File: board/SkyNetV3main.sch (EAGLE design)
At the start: 61 parts, among them IC1 HC_05, IC2 RF4463PRO, IC3 LPC1768, IC4 BCX17, IC5 TPS63001, IC6 MCP73871-2CCI/ML, Q1 32.768KHz, Q2 12MHz, Q3 IRLM6402, Q4 BSS138, X1 BAT

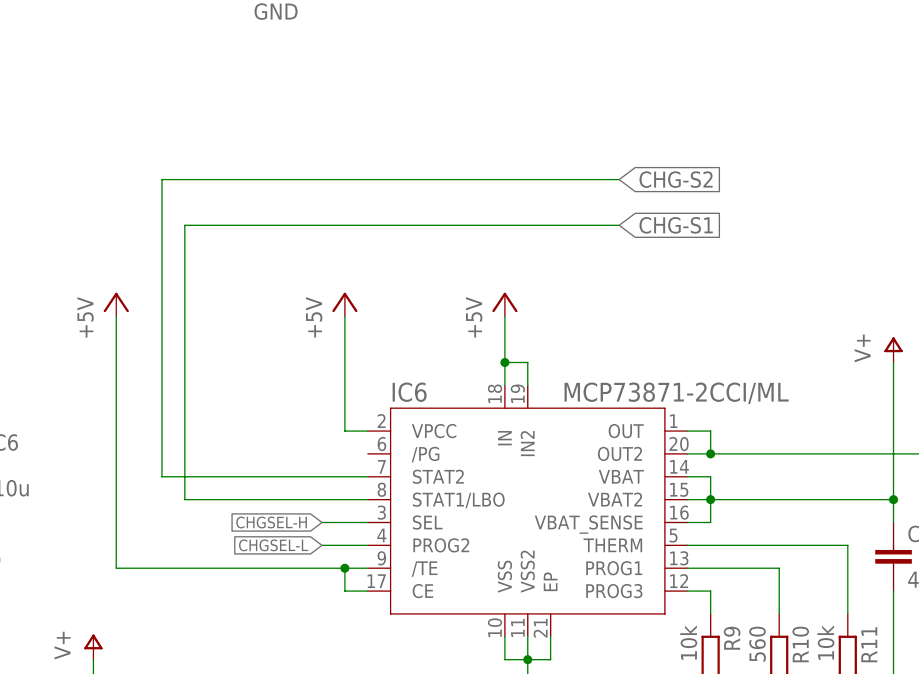
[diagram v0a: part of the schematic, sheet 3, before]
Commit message: layout improvements
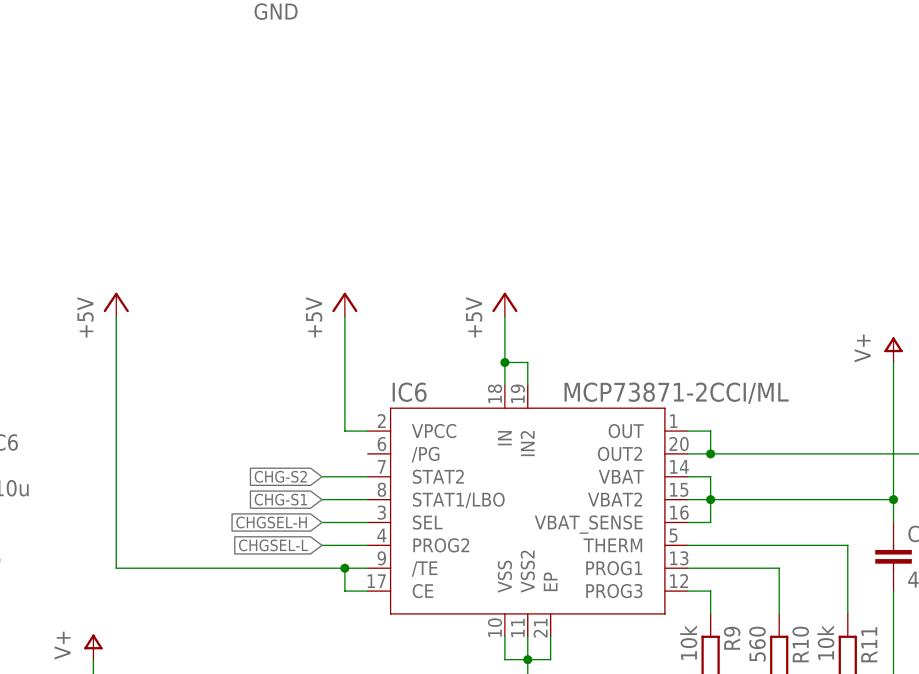
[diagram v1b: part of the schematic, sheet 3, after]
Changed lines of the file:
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@@
 <segment>
 <pinref part="IC6" gate="A" pin="STAT1/LBO"/>
-<wire x1="60.96" y1="93.98" x2="40.64" y2="93.98" width="0.1524" layer="91"/>
-<wire x1="40.64" y1="93.98" x2="40.64" y2="124.46" width="0.1524" layer="91"/>
-<wire x1="88.9" y1="124.46" x2="40.64" y2="124.46" width="0.1524" layer="91"/>
-<label x="88.9" y="124.46" size="1.778" layer="95" xref="yes"/>
+<wire x1="60.96" y1="93.98" x2="55.88" y2="93.98" width="0.1524" layer="91"/>
+<label x="55.88" y="93.98" size="1.27" layer="95" rot="R180" xref="yes"/>
 </segment>
 </net>
@@
 <segment>
 <pinref part="IC6" gate="A" pin="STAT2"/>
-<wire x1="60.96" y1="96.52" x2="38.1" y2="96.52" width="0.1524" layer="91"/>
-<wire x1="38.1" y1="96.52" x2="38.1" y2="129.54" width="0.1524" layer="91"/>
-<label x="88.9" y="129.54" size="1.778" layer="95" rot="MR180" xref="yes"/>
-<wire x1="38.1" y1="129.54" x2="88.9" y2="129.54" width="0.1524" layer="91"/>
+<wire x1="60.96" y1="96.52" x2="55.88" y2="96.52" width="0.1524" layer="91"/>
+<label x="55.88" y="96.52" size="1.27" layer="95" rot="MR0" xref="yes"/>
 </segment>
 </net>
